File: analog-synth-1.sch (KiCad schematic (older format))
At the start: 0 parts

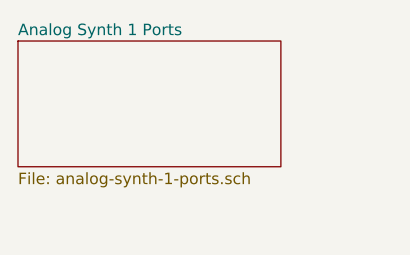
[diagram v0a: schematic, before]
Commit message: Begin working on ports
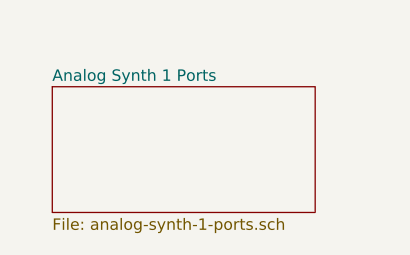
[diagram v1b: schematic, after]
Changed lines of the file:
@@
 EESchema Schematic File Version 4
+LIBS:analog-synth-1-cache
 EELAYER 26 0
 EELAYER END
@@
 $EndDescr
 $Sheet
-S 1200 1200 1150 550
+S 1350 1400 1150 550
 U 5C85AB83
 F0 "Analog Synth 1 Ports" 50
